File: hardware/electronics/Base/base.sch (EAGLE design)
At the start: 23 parts, among them IC1 7805T, IC2 74LS595D

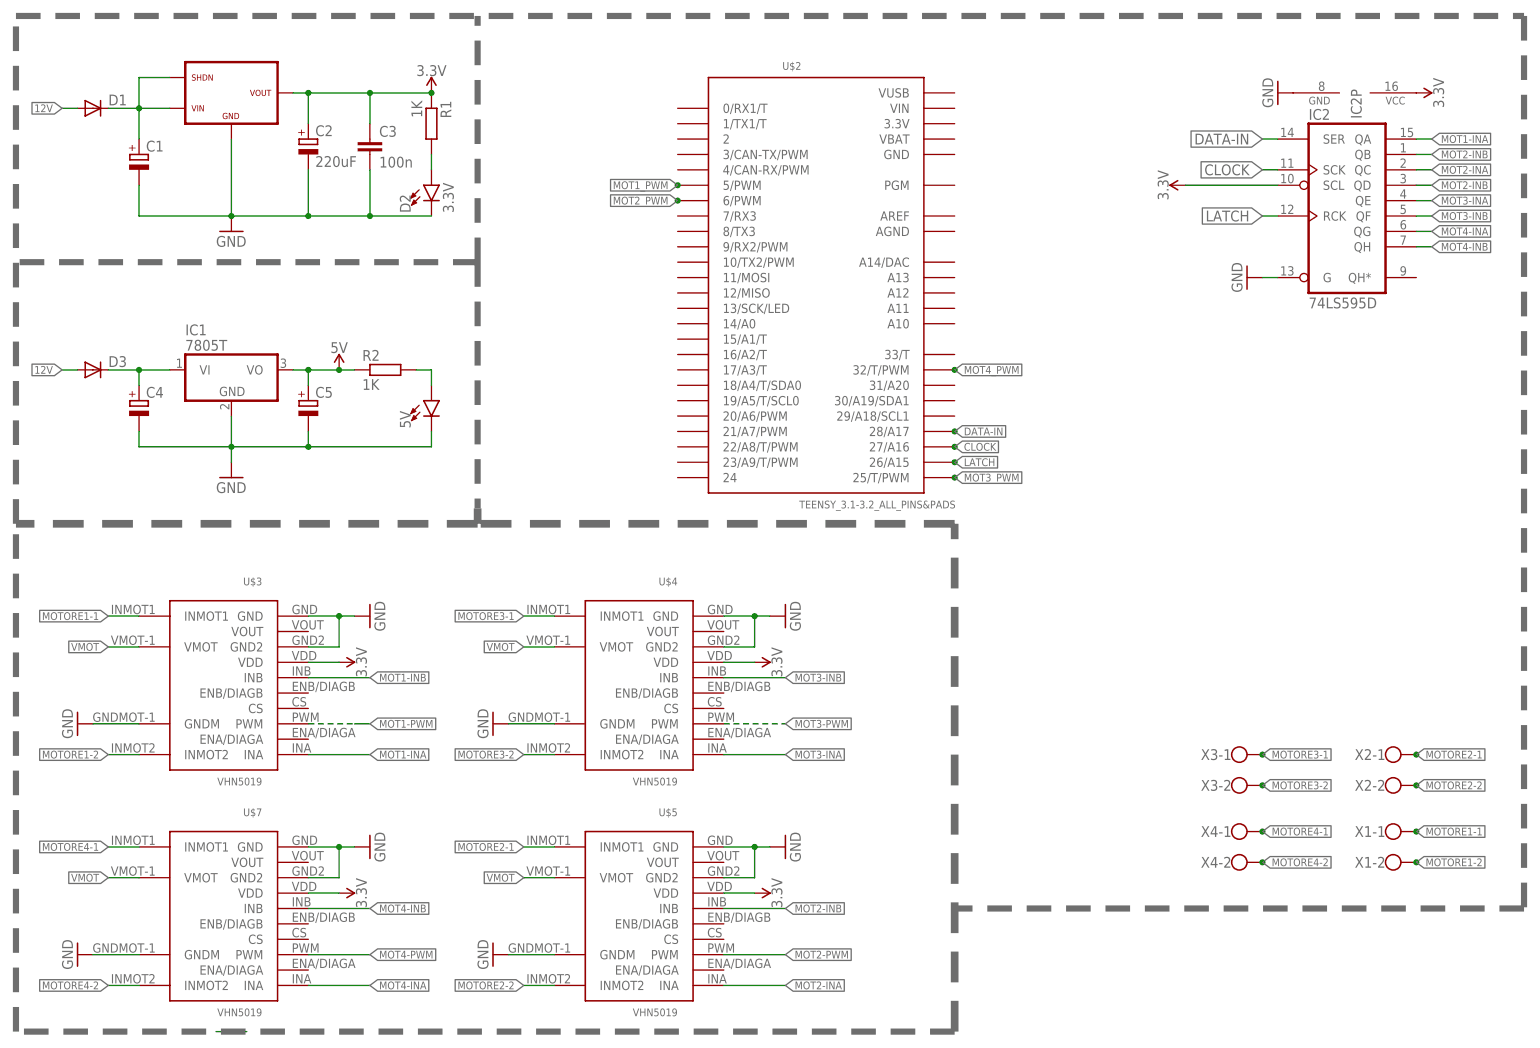
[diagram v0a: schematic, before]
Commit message: Base aggiornata
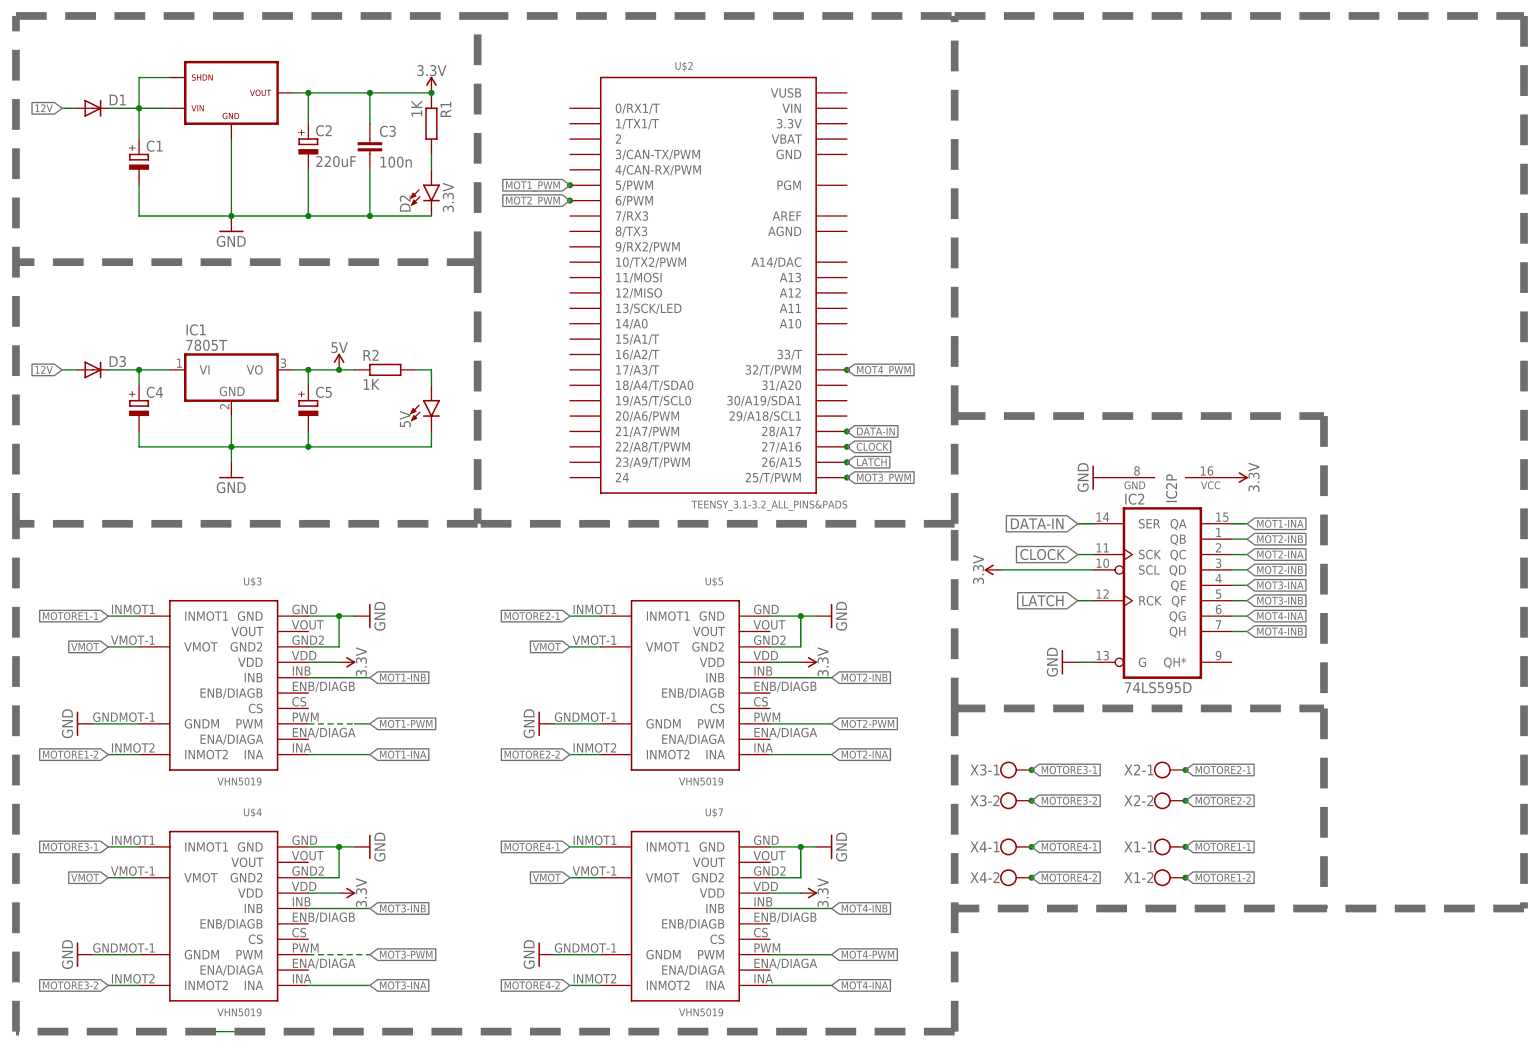
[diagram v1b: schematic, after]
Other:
- note added: "Motor driver VHN5019"
- note added: "Pin motori"
- note added: "Shift register"
- note added: "Teensy 3.2"
- moved on the sheet: IC2, IC2P, U$2, U$4, U$5, U$7, X1-1, X1-2, X2-1, X2-2, X3-1, X3-2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

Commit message: base
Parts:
- added B1: SD_MMC_CARDSD_PCB, SparkFun-Boards:SD_MMC_CARDSD_PCB
- added IC3: 74LS595D, 74xx-us:74LS595D
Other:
- note added: "Shift register motori"
- note removed: "Shift register"
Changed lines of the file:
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@@
 <part name="X3" library="con-wago-500" library_urn="urn:adsk.eagle:library:195" deviceset="W237-102" device="" package3d_urn="urn:adsk.eagle:package:10688/1"/>
 <part name="X4" library="con-wago-500" library_urn="urn:adsk.eagle:library:195" deviceset="W237-102" device="" package3d_urn="urn:adsk.eagle:package:10688/1"/>
+<part name="FRAME2" library="frames" library_urn="urn:adsk.eagle:library:229" deviceset="A4L-LOC" device=""/>
+<part name="IC3" library="74xx-us" library_urn="urn:adsk.eagle:library:88" deviceset="74*595" device="D" package3d_urn="urn:adsk.eagle:package:2918/1" technology="LS"/>
+<part name="B1" library="SparkFun-Boards" deviceset="SD_MMC_CARD" device="SD_PCB"/>
 </parts>
 <sheets>
@@
 <wire x1="55.88" y1="81.28" x2="55.88" y2="111.76" width="1.27" layer="96" style="longdash"/>
 <wire x1="55.88" y1="81.28" x2="116.84" y2="81.28" width="1.27" layer="96" style="longdash"/>
-<text x="81.28" y="124.46" size="2.54" layer="99">Shift register</text>
+<text x="81.28" y="124.46" size="2.54" layer="99">Shift register motori</text>
 <wire x1="55.88" y1="111.76" x2="55.88" y2="129.54" width="1.27" layer="96" style="longdash"/>
 <wire x1="55.88" y1="129.54" x2="116.84" y2="129.54" width="1.27" layer="96" style="longdash"/>
@@
 </nets>
 </sheet>
+<sheet>
+<plain>
+</plain>
+<instances>
+<instance part="FRAME2" gate="G$1" x="0" y="0"/>
+<instance part="IC3" gate="A" x="66.04" y="116.84"/>
+<instance part="B1" gate="G$1" x="121.92" y="116.84"/>
+</instances>
+<busses>
+</busses>
+<nets>
+</nets>
+</sheet>
